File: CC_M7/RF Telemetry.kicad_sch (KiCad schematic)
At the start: 26 parts, among them J15 Conn_02x05_Odd_Even, J9 Antenna, U6 nRF52820-QDxx, U7 NRF21540-QDAA-R7, Y2 32MHz

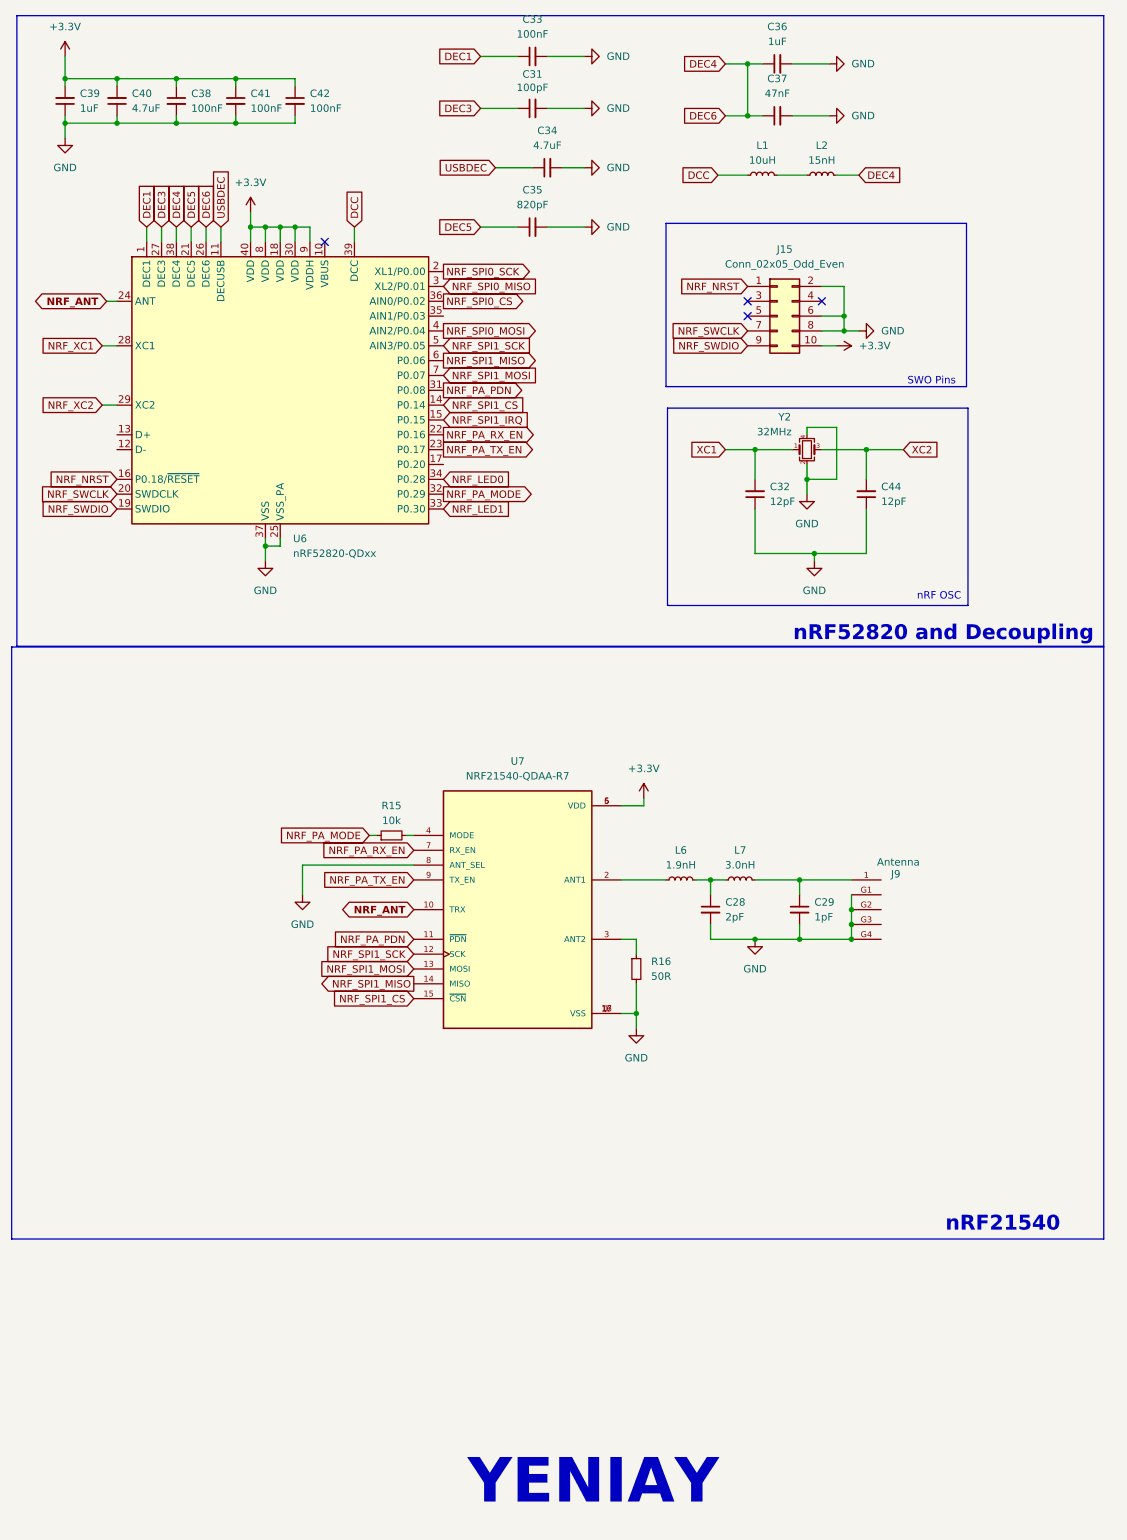
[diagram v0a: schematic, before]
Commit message: final schematic 6 warning
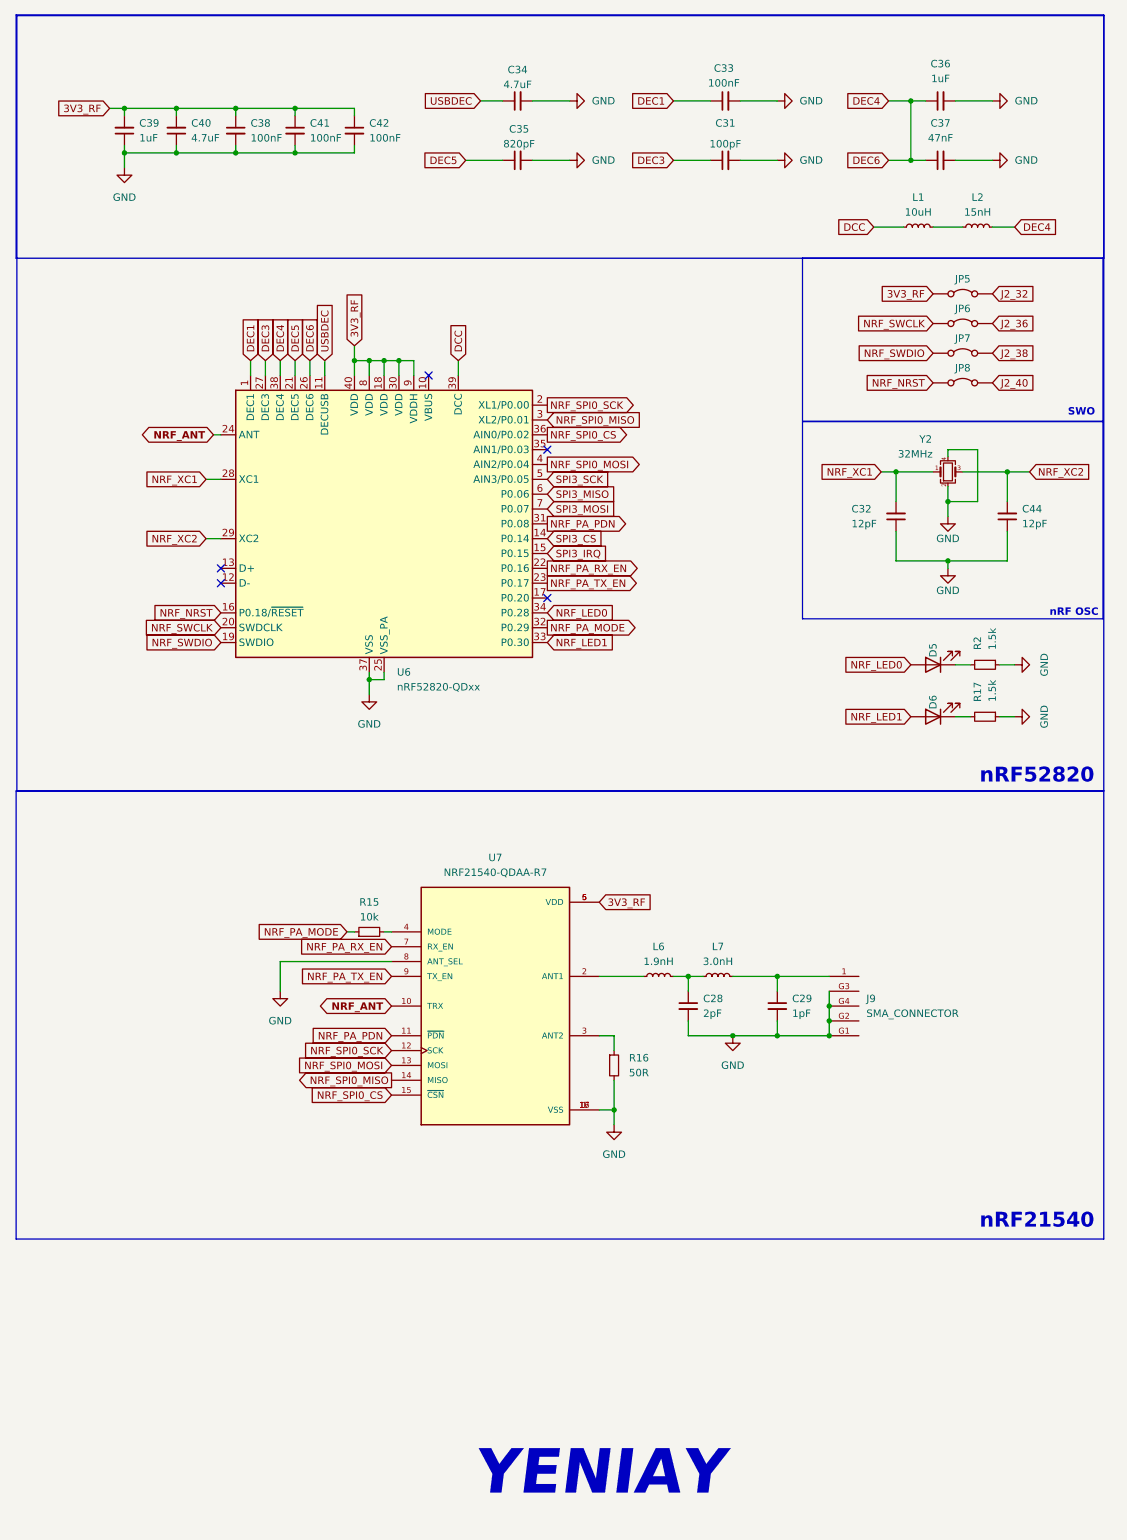
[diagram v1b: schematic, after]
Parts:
- removed J15: Conn_02x05_Odd_Even, symbol Connector_Generic:Conn_02x05_Odd_Even
- added D5, D6: LED, symbol Device:LED
- added JP5, JP6, JP7, JP8: SWDIO, symbol Jumper:Jumper_2_Bridged
- added R17, R2: 1.5k, symbol Device:R_Small
- J9: value Antenna -> SMA_CONNECTOR
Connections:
- net XC1 is gone; now on net NRF_XC1: C32.2, Y2.1
- net XC2 is gone; now on net NRF_XC2: C44.2, Y2.3
- net GND: now also R17.1, R2.1
- net NRF_LED0: now also D5.2 (A)
- net NRF_LED1: now also D6.2 (A)
- net NRF_NRST: now also JP8.1 (A)
- net NRF_SPI0_CS: now also U7.15 (~{CSN})
- net NRF_SPI0_MISO: now also U7.14 (MISO)
- net NRF_SPI0_MOSI: now also U7.13 (MOSI)
- net NRF_SPI0_SCK: now also U7.12 (SCK)
- net NRF_SWCLK: now also JP6.1 (A)
- net NRF_SWDIO: now also JP7.1 (A)
- net +3.3V renamed 3V3_RF
- net 3V3_RF: now also JP5.1 (A)
- net NRF_SPI1_CS renamed SPI3_CS
- net SPI3_CS: no longer U7.15 (~{CSN})
- net NRF_SPI1_IRQ renamed SPI3_IRQ
- net NRF_SPI1_MISO renamed SPI3_MISO
- net SPI3_MISO: no longer U7.14 (MISO)
- net NRF_SPI1_MOSI renamed SPI3_MOSI
- net SPI3_MOSI: no longer U7.13 (MOSI)
- net NRF_SPI1_SCK renamed SPI3_SCK
- net SPI3_SCK: no longer U7.12 (SCK)
- new net: D6.1 (K), R17.2
- new net: D5.1 (K), R2.2
- new net J2_32: JP5.2 (B)
- new net J2_36: JP6.2 (B)
- new net J2_38: JP7.2 (B)
- new net J2_40: JP8.2 (B)
- no-connect marks 4 -> 5
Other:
- note added: "SWO"
- note added: "nRF52820"
- note removed: "SWO Pins"
- note removed: "nRF52820 and Decoupling"
- moved on the sheet: C28, C29, C31, C32, C33, C34, C35, C36, C37, C38, C39, C40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
